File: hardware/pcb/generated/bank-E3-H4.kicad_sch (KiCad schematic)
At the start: 34 parts, among them U26 SK9822-EC20, U27 SK9822-EC20, U28 SK9822-EC20, U29 SK9822-EC20, U30 SK9822-EC20, U31 SK9822-EC20, U32 SK9822-EC20, U33 SK9822-EC20, U4 TCA9554DWR

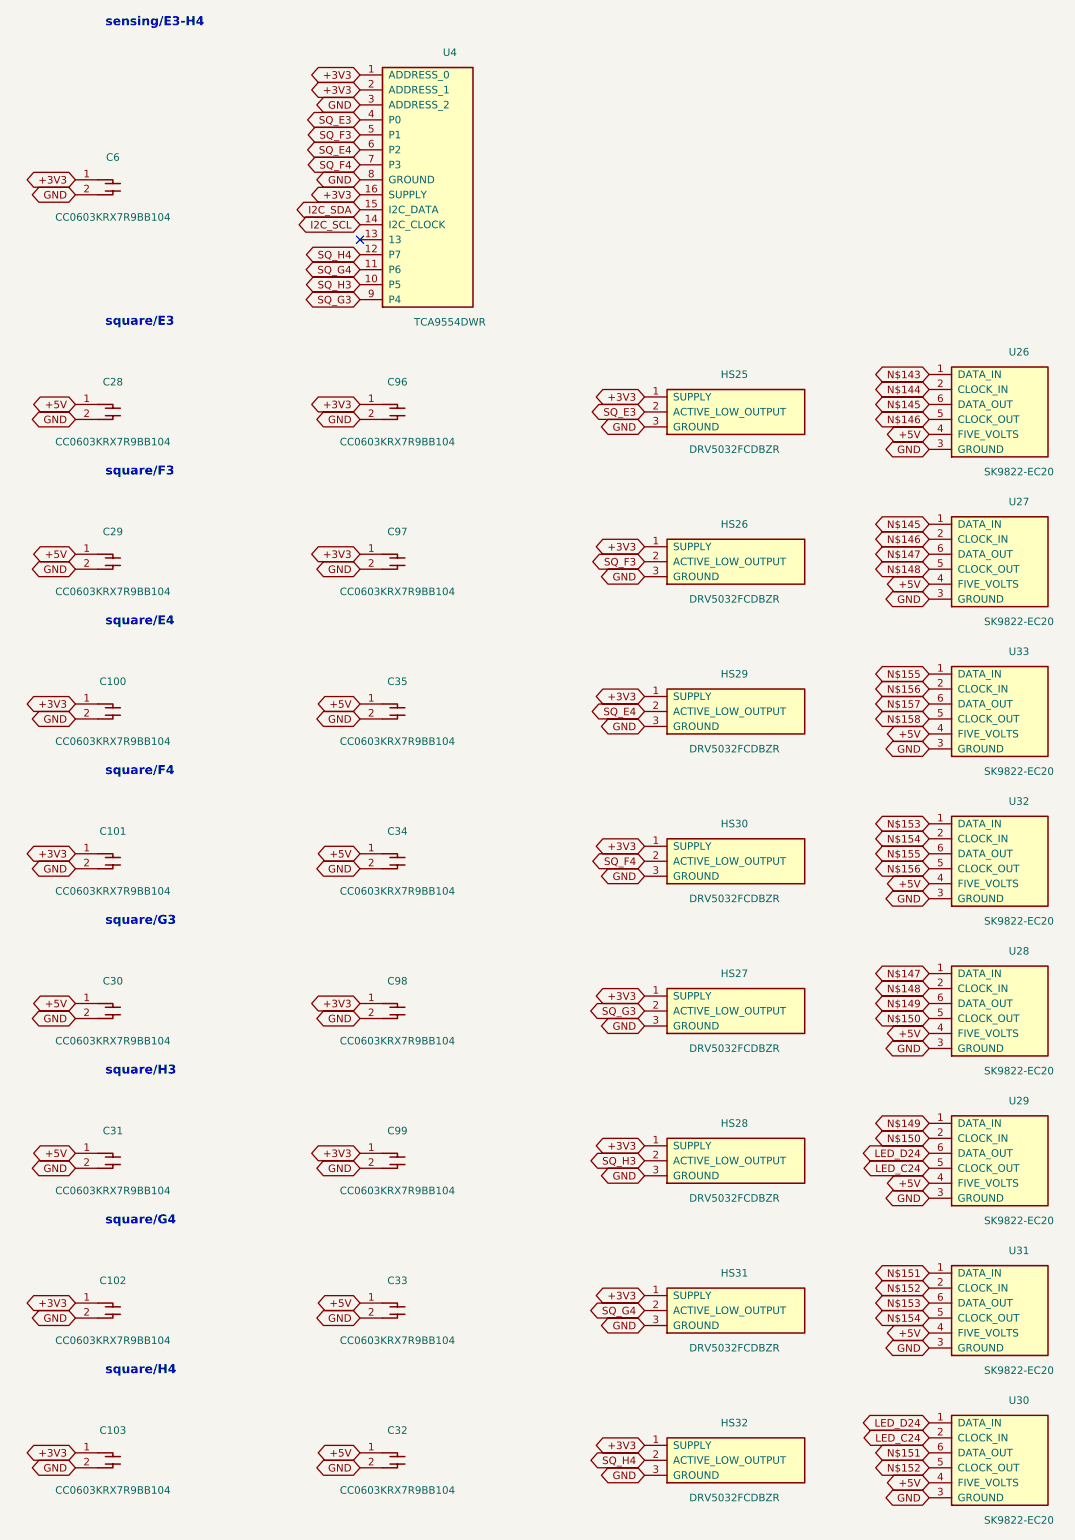
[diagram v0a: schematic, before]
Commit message: chore(pcb): regenerate KiCad, SPICE and review output
Generated by `just pcb` from the committed definition; not hand-edited.
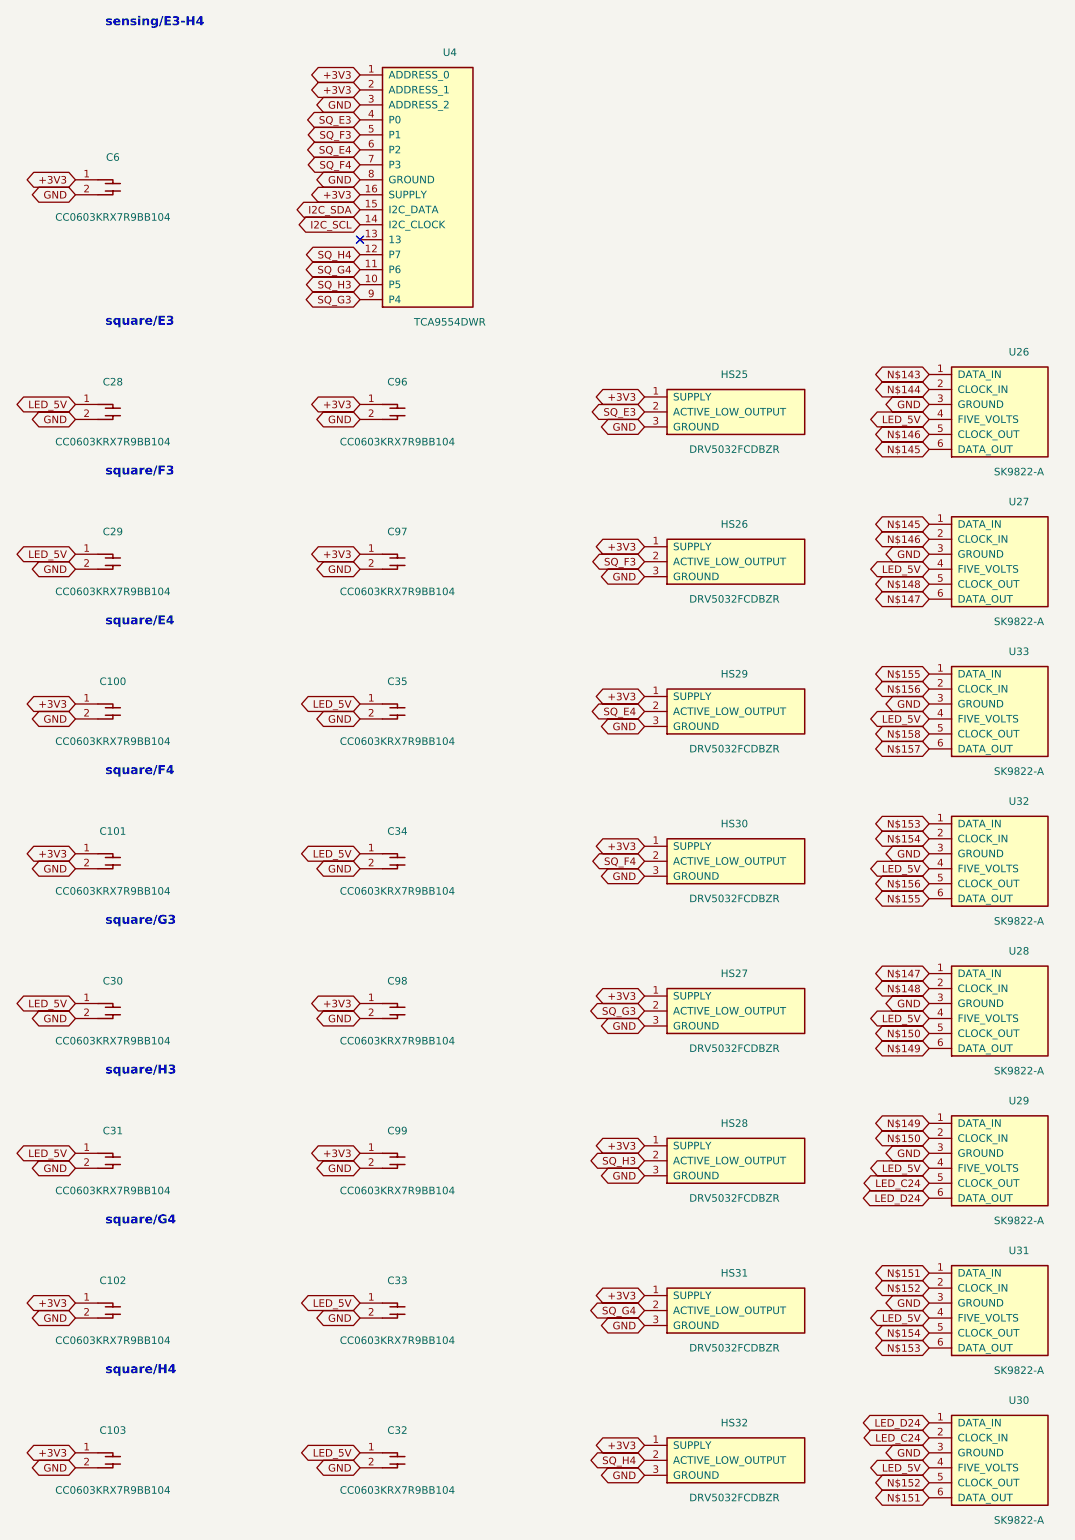
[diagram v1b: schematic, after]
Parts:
- U26, U27, U28, U29, U30, U31, U32, U33: value SK9822-EC20 -> SK9822-A
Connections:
- net +5V renamed LED_5V
